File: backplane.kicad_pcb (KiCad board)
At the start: 2 copper layers, 93.9 x 83.8 mm, 63 parts, among them J1 I2C, J2 I2C, J3 SER, J4 PWR, J5 PWR, J6 FAN, J7 PPS, Q4 Q_NMOS_GSD, Q5 Q_PMOS_GSD, SW1 SW_Push, U1 Raspberry_Pi_2_3, U2 IC880A-SPI, U3 SHT21, U4 MP1584_MODULE, U5 MCP3425A0T-E/CH

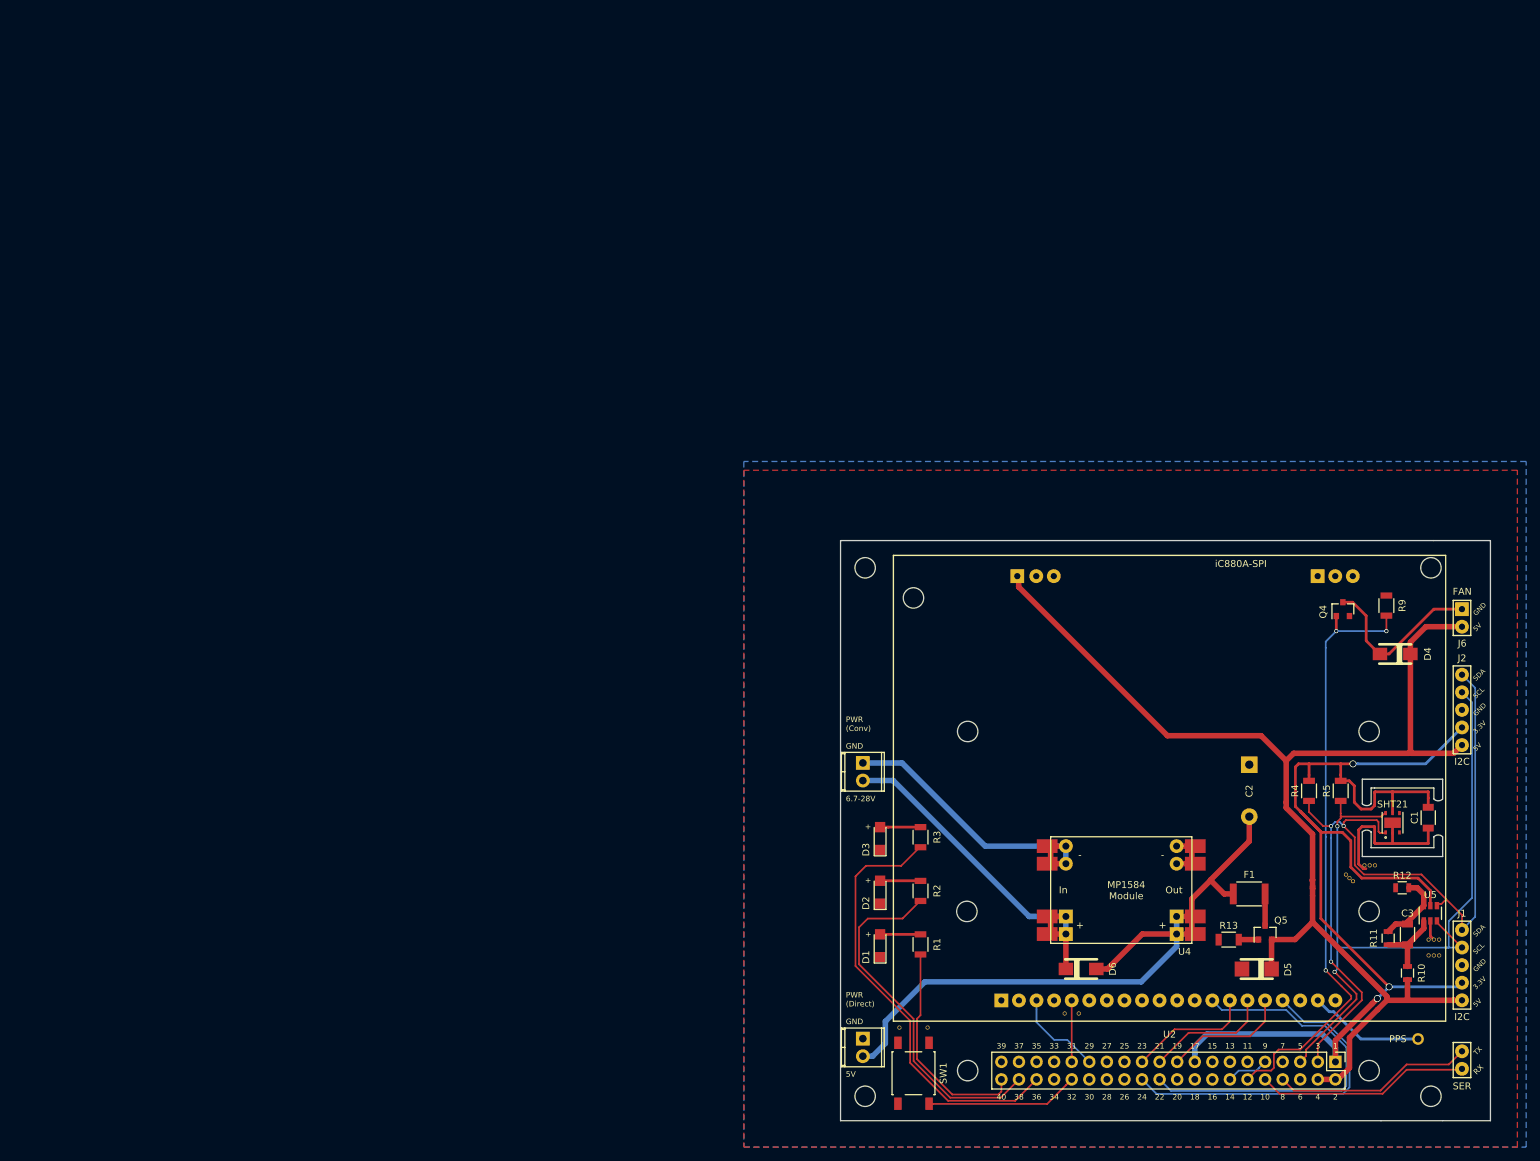
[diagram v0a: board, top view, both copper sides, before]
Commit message: modified for base48, different supply, layout
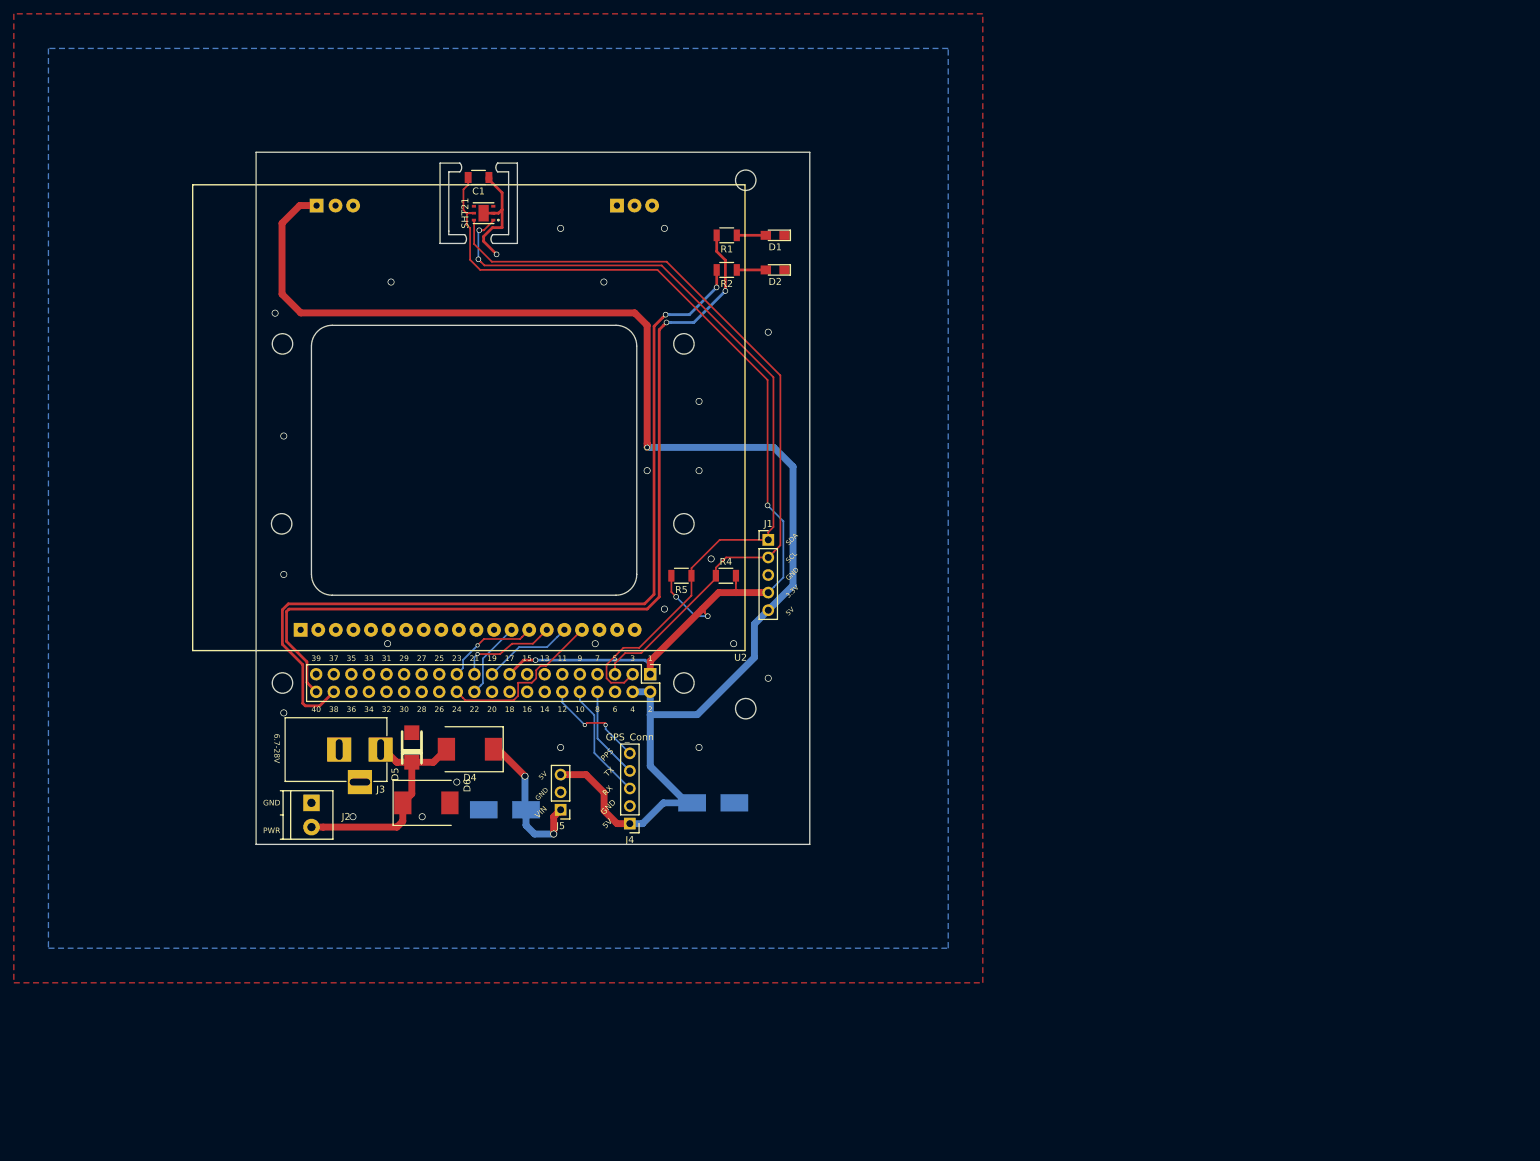
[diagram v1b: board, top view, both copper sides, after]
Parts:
- removed D3: LED_Red, LEDs:LED_1206
- removed F1: Polyfuse, Capacitors_SMD:C_1812
- removed J6: FAN, headers:header_1x2_marked
- removed J7: PPS, headers:header_1x1_unmarked
- removed Q4: Q_NMOS_GSD, TO_SOT_Packages_SMD:SOT-23
- removed Q5: Q_PMOS_GSD, TO_SOT_Packages_SMD:SOT-23
- removed R10, R11, R12: R, Resistors_SMD:R_0805
- removed R13, R9: R, Resistors_SMD:R_1206
- removed R3: 220Ω 1/8W, Resistors_SMD:R_1206
- removed the REF** at (126.0, 78.4)
- removed the REF** at (119.0, 150.4)
- removed the REF** at (119.0, 74.0)
- removed the REF** at (200.4, 127.8)
- removed the REF** at (149.9, 138.4)
- removed the REF** at (201.2, 127.8)
- removed the REF** at (201.9, 127.8)
- removed the REF** at (200.4, 130.0)
- removed the REF** at (201.2, 130.0)
- removed the REF** at (201.9, 130.0)
- removed the REF** at (191.1, 117.0)
- removed the REF** at (191.9, 117.0)
- removed the REF** at (124.0, 140.5)
- removed the REF** at (147.8, 138.4)
- removed the REF** at (128.0, 140.5)
- removed the REF** at (189.5, 119.3)
- removed the REF** at (188.5, 118.4)
- removed the REF** at (189.0, 118.9)
- removed the REF** at (192.7, 117.0)
- removed SW1: SW_Push, buttons:SW_Mikroshop
- removed U4: MP1584_MODULE, regulators:MP1584_MODULE_ZVEPOWER
- removed U5: MCP3425A0T-E/CH, TO_SOT_Packages_SMD:SOT-23-6
- C2: footprint capacitor-unmarked:CAP_UNMARKED -> Capacitors_SMD:CP_Elec_8x10; moved to B.Cu
- C3: footprint Capacitors_SMD:C_1206 -> Capacitors_SMD:CP_Elec_8x10; moved to B.Cu
- D1, D2: footprint LEDs:LED_1206 -> LEDs:LED_0805_HandSoldering
- D4: value D -> D_Schottky; footprint DO214:DO-214AC -> Diodes_SMD:D_SMC
- D6: value D -> D_TVS; footprint DO214:DO-214AC -> Diodes_SMD:D_SMC
- J1: footprint headers:header_1x5_unmarked -> Socket_Strips:Socket_Strip_Straight_1x05_Pitch2.54mm
- J2: value I2C -> PWR; footprint headers:header_1x5_unmarked -> TerminalBlock_Phoenix:TerminalBlock_Phoenix_PT-3.5mm_2pol
- J3: value SER -> Barrel_Jack; footprint headers:header_1x2_unmarked -> Connectors:BARREL_JACK
- J4: value PWR -> GPS_Conn; footprint Connectors_Terminal_Blocks:TerminalBlock_Pheonix_MPT-2.54mm_2pol -> Socket_Strips:Socket_Strip_Straight_1x05_Pitch2.54mm
- J5: value PWR -> REG_Conn; footprint Connectors_Terminal_Blocks:TerminalBlock_Pheonix_MPT-2.54mm_2pol -> Pin_Headers:Pin_Header_Straight_1x03_Pitch2.54mm
- moved J2 167.3 mm to (39.0, 108.0), turned to 270 degrees
- moved C1 165.5 mm to (63.1, 17.6), turned to 180 degrees
- moved J3 162.2 mm to (49.0, 100.3)
- moved U3 158.1 mm to (63.9, 22.8), turned to 90 degrees
- moved D4 134.4 mm to (61.9, 100.2)
- moved D5 126.2 mm to (53.5, 100.0), turned to 90 degrees
- moved J1 115.0 mm to (105.0, 70.0)
- moved U2 114.5 mm to (61.7, 52.4)
- moved REF** 113.7 mm to (101.7, 18.0)
- moved REF** 113.7 mm to (34.8, 90.7)
- moved REF** 113.7 mm to (34.7, 67.7)
- moved REF** 113.7 mm to (101.7, 94.4)
- moved REF** 113.7 mm to (92.8, 67.7)
- moved REF** 113.7 mm to (92.8, 41.7)
- moved REF** 113.7 mm to (34.8, 41.7)
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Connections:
- C3 pad 1: Net-(C3-Pad1) -> GND
- C3 pad 2: Net-(C3-Pad2) -> 5V
- D4 pad 1: 5V -> Net-(C2-Pad2)
- D4 pad 2: Net-(D4-Pad2) -> VIN
- D5 pad 1: 5V -> VIN
- D6 pad 1: Net-(D6-Pad1) -> VIN
- D6 pad 2: Net-(C2-Pad2) -> GND
- J2 pad 1: SDA -> GND
- J2 pad 2: SCL -> VIN
- J3 pad 1: TX -> VIN
- J3 pad 2: RX -> GND
- J4 pad 1: GND -> 5V
- J4 pad 2: Net-(C2-Pad2) -> GND
- J5 pad 1: Net-(J5-Pad1) -> Net-(C2-Pad2)
- J5 pad 2: Net-(D6-Pad1) -> GND
- R4 pad 2: SDA -> SCL
- R5 pad 2: SCL -> SDA
- U1 pad 11: (no net) -> Net-(U1-Pad11)
- U1 pad 12: FAN -> PPS
- U1 pad 13: (no net) -> Net-(U1-Pad13)
- U1 pad 15: (no net) -> Net-(U1-Pad15)
- U1 pad 16: (no net) -> Net-(U1-Pad16)
- U1 pad 18: (no net) -> Net-(U1-Pad18)
- U1 pad 26: (no net) -> Net-(U1-Pad26)
- U1 pad 27: (no net) -> Net-(U1-Pad27)
- U1 pad 28: (no net) -> Net-(U1-Pad28)
- U1 pad 29: GPS_RST -> Net-(U1-Pad29)
- U1 pad 31: GPS_SUP -> Net-(U1-Pad31)
- U1 pad 32: BTN -> Net-(U1-Pad32)
- U1 pad 33: (no net) -> Net-(U1-Pad33)
- U1 pad 35: (no net) -> Net-(U1-Pad35)
- U1 pad 36: LED3 -> Net-(U1-Pad36)
- U1 pad 37: (no net) -> Net-(U1-Pad37)
- U1 pad 6: (no net) -> Net-(U1-Pad6)
- U1 pad 7: (no net) -> Net-(U1-Pad7)
- U2 pad 10: (no net) -> Net-(U2-Pad10)
- U2 pad 11: (no net) -> Net-(U2-Pad11)
- U2 pad 18: (no net) -> Net-(U2-Pad18)
- U2 pad 19: PPS -> Net-(U2-Pad19)
- U2 pad 2: (no net) -> Net-(U2-Pad2)
- U2 pad 23: (no net) -> Net-(U2-Pad23)
- U2 pad 25: (no net) -> Net-(U2-Pad25)
- U2 pad 26: (no net) -> Net-(U2-Pad26)
- U2 pad 3: GPS_RST -> Net-(U2-Pad3)
- U2 pad 4: (no net) -> Net-(U2-Pad4)
- U2 pad 5: GPS_SUP -> Net-(U2-Pad5)
- U2 pad 6: (no net) -> Net-(U2-Pad6)
- U2 pad 7: (no net) -> Net-(U2-Pad7)
- U2 pad 8: (no net) -> Net-(U2-Pad8)
- U2 pad 9: (no net) -> Net-(U2-Pad9)
- U3 pad 3: (no net) -> Net-(U3-Pad3)
- U3 pad 4: (no net) -> Net-(U3-Pad4)
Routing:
- net LED1: track 31.6 -> 127.1 mm, vias 0 -> 2
- net FAN: track 87.9 -> 0.00 mm, vias 3 -> 0
- net Net-(C2-Pad2): track 100.7 -> 21.8 mm, vias 0 -> 2
- net LED2: track 51.6 -> 127.5 mm, vias 0 -> 2
- net LED3: track 63.2 -> 0.00 mm
- net Net-(D6-Pad1): track 52.0 -> 0.00 mm
- net IC880A_RST: track 55.7 -> 11.2 mm
- net Net-(J5-Pad1): track 43.8 -> 0.00 mm
- net VIN: track 0.00 -> 33.6 mm
- net Net-(D4-Pad2): track 25.1 -> 0.00 mm
- net CE0: track 49.6 -> 24.6 mm
- net GND: track 40.3 -> 17.5 mm, vias 0 -> 24
- net BTN: track 22.3 -> 0.00 mm
- net 5V: track 185.2 -> 205.4 mm, vias 0 -> 1
- net TX: track 28.9 -> 13.4 mm
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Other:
- board size 93.9 x 83.8 mm -> 80 x 100 mm
- net class Power: trace_width 0.8 -> 1; via_drill 0.8 -> 0.6
- board text added: "PPS"
- board text added: "PWR"
- board text added: "VIN"
- board text added: "iC880A Backplane v1.6a"
- board text added: "original by coredump.ch | modified by Adluc base48.cz"
- board text removed: "+"
- board text removed: "MP1584 Module"
- board text removed: "PWR (Conv)"
- board text removed: "PWR (Direct)"
- board text removed: "coredump.ch 2018"
- board text removed: "https://github.com/dbrgn/ic880a-backplane Designed & assembled in Switzerland"
- board text removed: "iC880A Backplane v1.6"
- board text removed: "iC880A-SPI"
